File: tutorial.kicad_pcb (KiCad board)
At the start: 2 copper layers, 178.2 x 165.7 mm, 73 parts

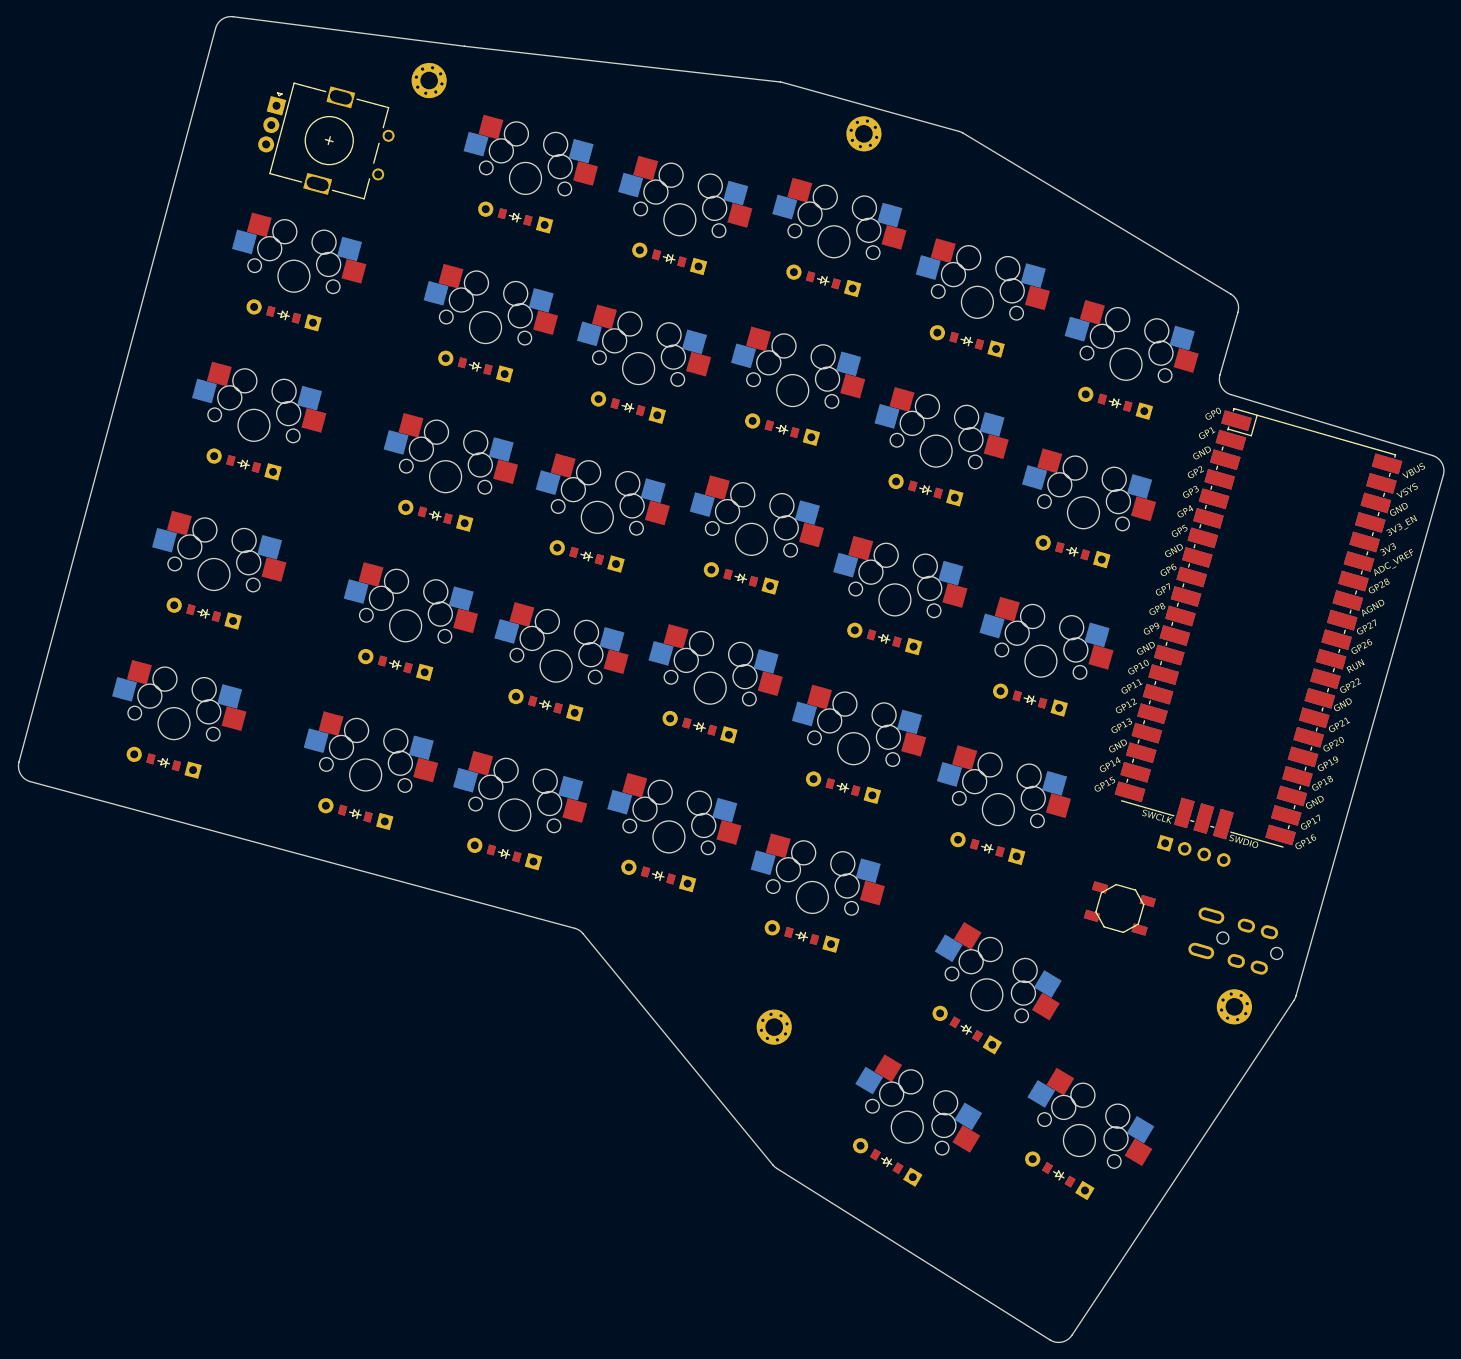
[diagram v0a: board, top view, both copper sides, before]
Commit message: routing done!
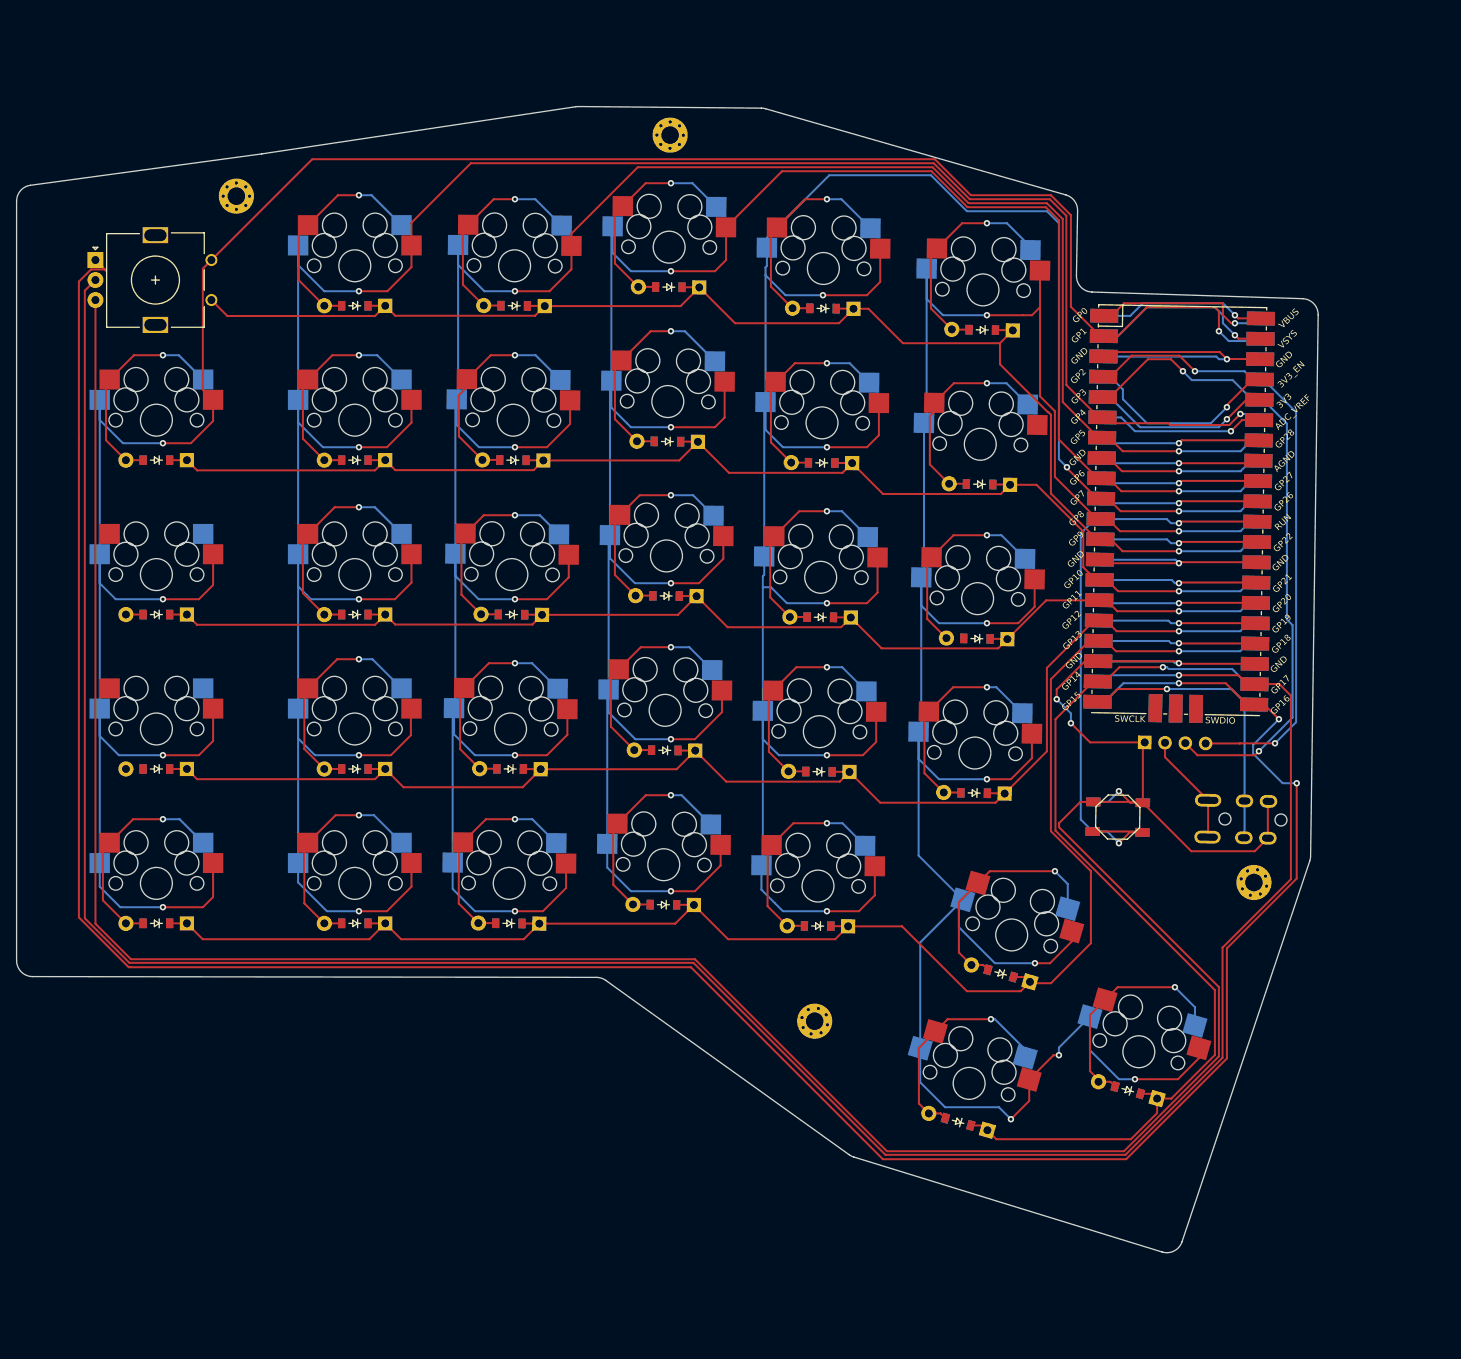
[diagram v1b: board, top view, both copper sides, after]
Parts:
- moved _5 28.1 mm to (118.9, 99.1), turned to 0 degrees
- moved ROT1 27.8 mm to (108.9, 109.7), turned to 0 degrees
- moved S4 24.9 mm to (108.9, 127.1), turned to 0 degrees
- moved _4 24.2 mm to (173.1, 91.5), turned to -0.5 degrees
- moved D4 24.1 mm to (108.9, 132.1), turned to 180 degrees
- moved S9 24.0 mm to (133.7, 107.8), turned to 0 degrees
- moved D9 22.9 mm to (133.7, 112.8), turned to 180 degrees
- moved S3 22.3 mm to (108.9, 146.4), turned to 0 degrees
- moved D3 21.8 mm to (108.9, 151.4), turned to 180 degrees
- moved S14 21.4 mm to (153.6, 107.8), turned to -0.5 degrees
- moved S19 20.6 mm to (173.0, 105.5), turned to -0.5 degrees
- moved S2 20.6 mm to (108.9, 165.7), turned to 0 degrees
- moved D2 20.4 mm to (108.9, 170.7), turned to 180 degrees
- moved D14 20.3 mm to (153.6, 112.8), turned to 179.5 degrees
- moved D1 20.2 mm to (108.9, 190.0), turned to 180 degrees
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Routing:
- net GND: track 0.00 -> 451.7 mm, vias 0 -> 7
- net GP4: track 0.00 -> 328.0 mm, vias 0 -> 6
- net GP1: track 0.00 -> 323.7 mm, vias 0 -> 5
- net GP16: track 0.00 -> 321.9 mm, vias 0 -> 3
- net GP17: track 0.00 -> 313.2 mm, vias 0 -> 1
- net GP5: track 0.00 -> 308.7 mm, vias 0 -> 6
- net GP8: track 0.00 -> 300.1 mm, vias 0 -> 8
- net GP6: track 0.00 -> 293.1 mm, vias 0 -> 6
- net GP7: track 0.00 -> 287.0 mm, vias 0 -> 7
- net GP13: track 0.00 -> 201.4 mm, vias 0 -> 1
- net GP12: track 0.00 -> 169.8 mm, vias 0 -> 1
- net GP9: track 0.00 -> 169.2 mm, vias 0 -> 1
- net GP10: track 0.00 -> 161.6 mm, vias 0 -> 1
- net GP11: track 0.00 -> 156.0 mm, vias 0 -> 1
- net GP14: track 0.00 -> 116.7 mm, vias 0 -> 1
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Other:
- board size 178.2 x 165.7 mm -> 162.7 x 143.3 mm
